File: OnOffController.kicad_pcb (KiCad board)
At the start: 2 copper layers, 16.5 x 23.9 mm, 33 parts, among them J1 S2B-PH-K-SLFSN, J2 Conn_01x02_Pin, J3 Conn_01x04_Pin, J4 Conn_01x04_Pin, J8 47589-0001, SW1 KMR211GLFS, U1 STM6601, U2 MCP73831-2-OT, U3 SPX3819M5-L

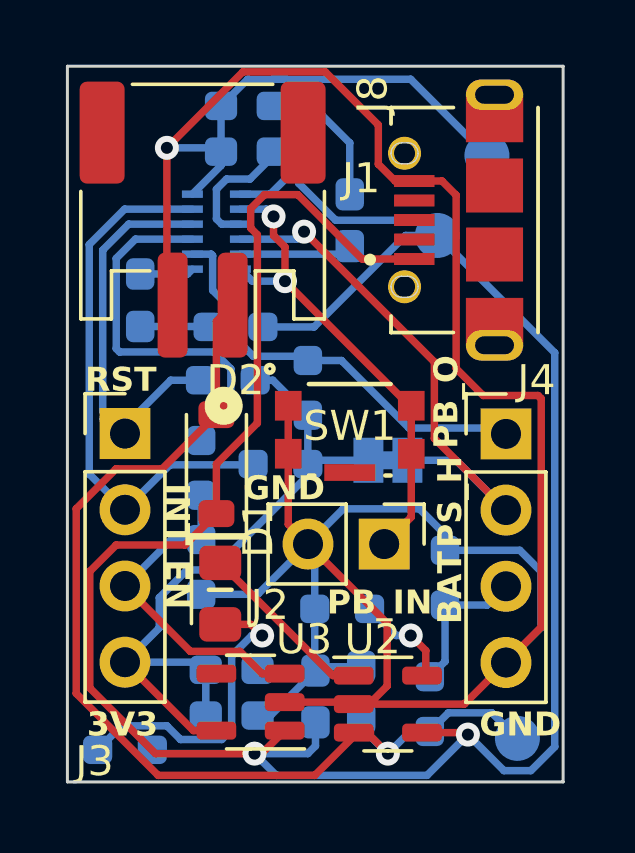
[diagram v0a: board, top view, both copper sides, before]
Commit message: Added BOM
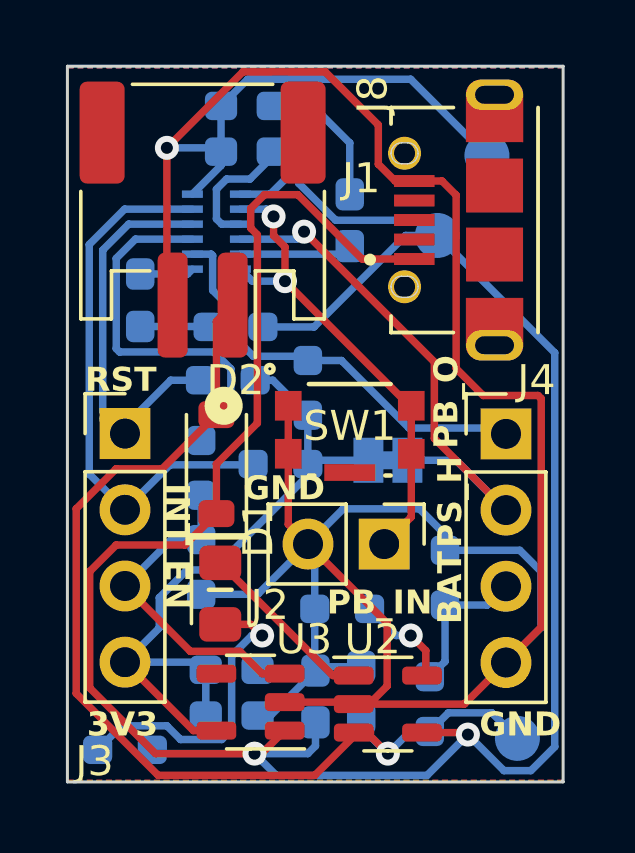
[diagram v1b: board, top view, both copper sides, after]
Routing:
- added copper zone on B.Cu, net GND
- added copper zone on F.Cu, net GND
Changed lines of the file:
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@@
   (segment (start 157.518 78.99) (end 159.389 78.99) (width 0.25) (layer "B.Cu") (net 28))
   (segment (start 159.389 78.99) (end 159.639 78.74) (width 0.25) (layer "B.Cu") (net 28))
+  (zone (net 2) (net_name "GND") (layers "F&B.Cu") (hatch edge 0.5)
+    (connect_pads (clearance 0.5))
+    (min_thickness 0.25) (filled_areas_thickness no)
+    (fill yes (thermal_gap 0.5) (thermal_bridge_width 0.5))
+    (polygon
+      (pts
+        (xy 151.765 73.279)
+        (xy 168.275 73.279)
+        (xy 168.275 97.028)
+        (xy 151.765 97.028)
+      )
+    )
+  )
 )
